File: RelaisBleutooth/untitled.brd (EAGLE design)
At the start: 160 x 100 mm, 3 parts

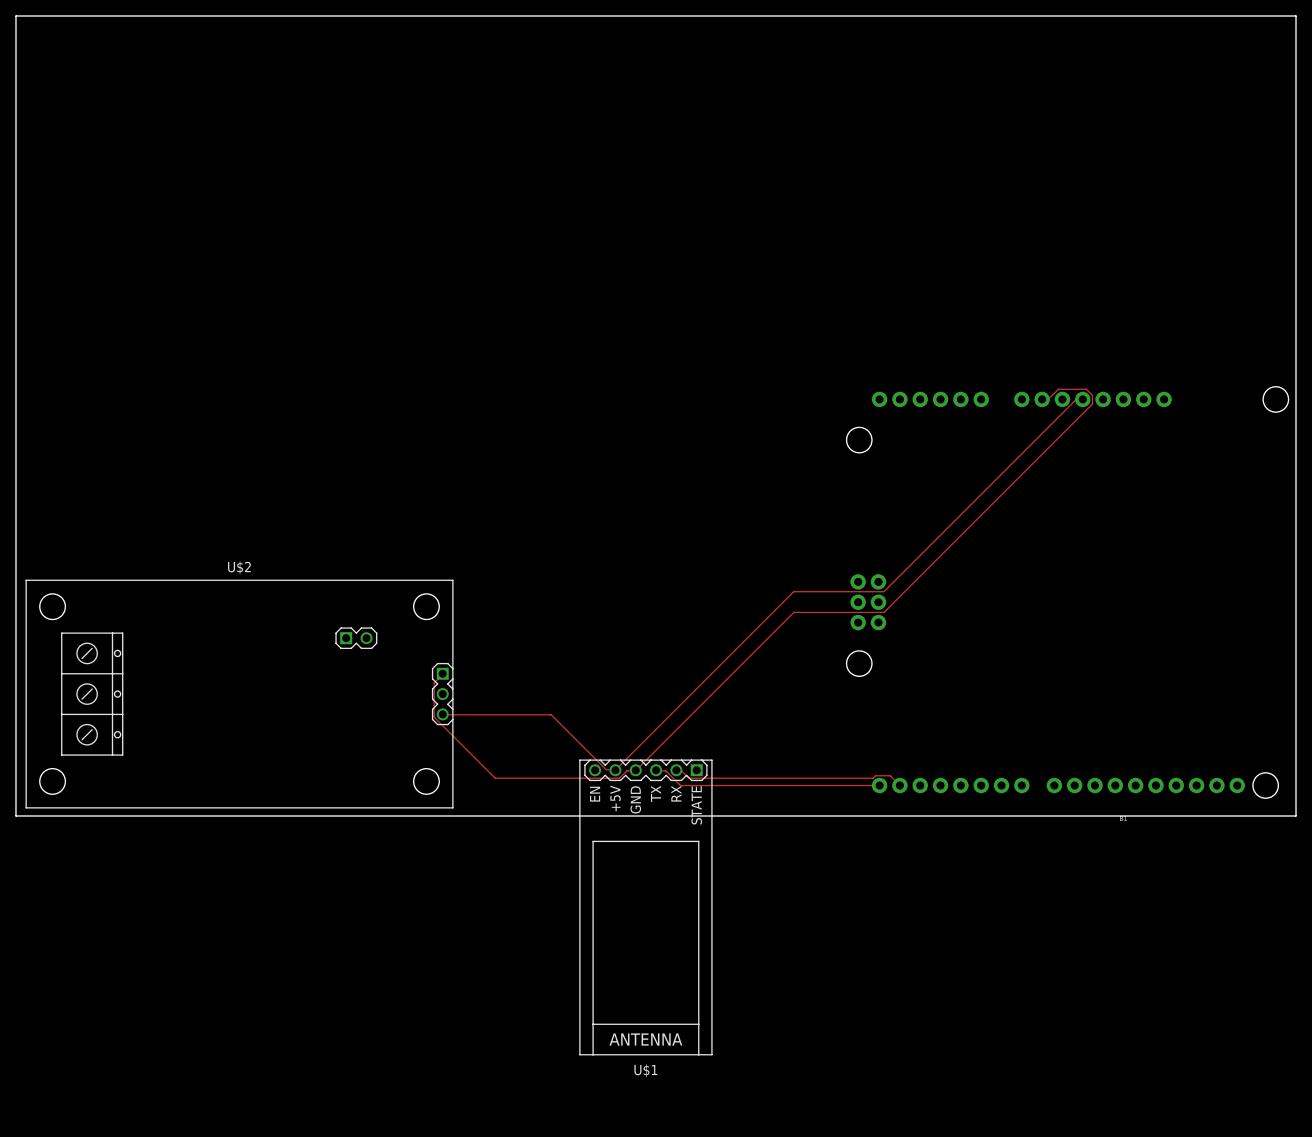
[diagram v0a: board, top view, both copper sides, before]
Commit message: Mise a jour des schema
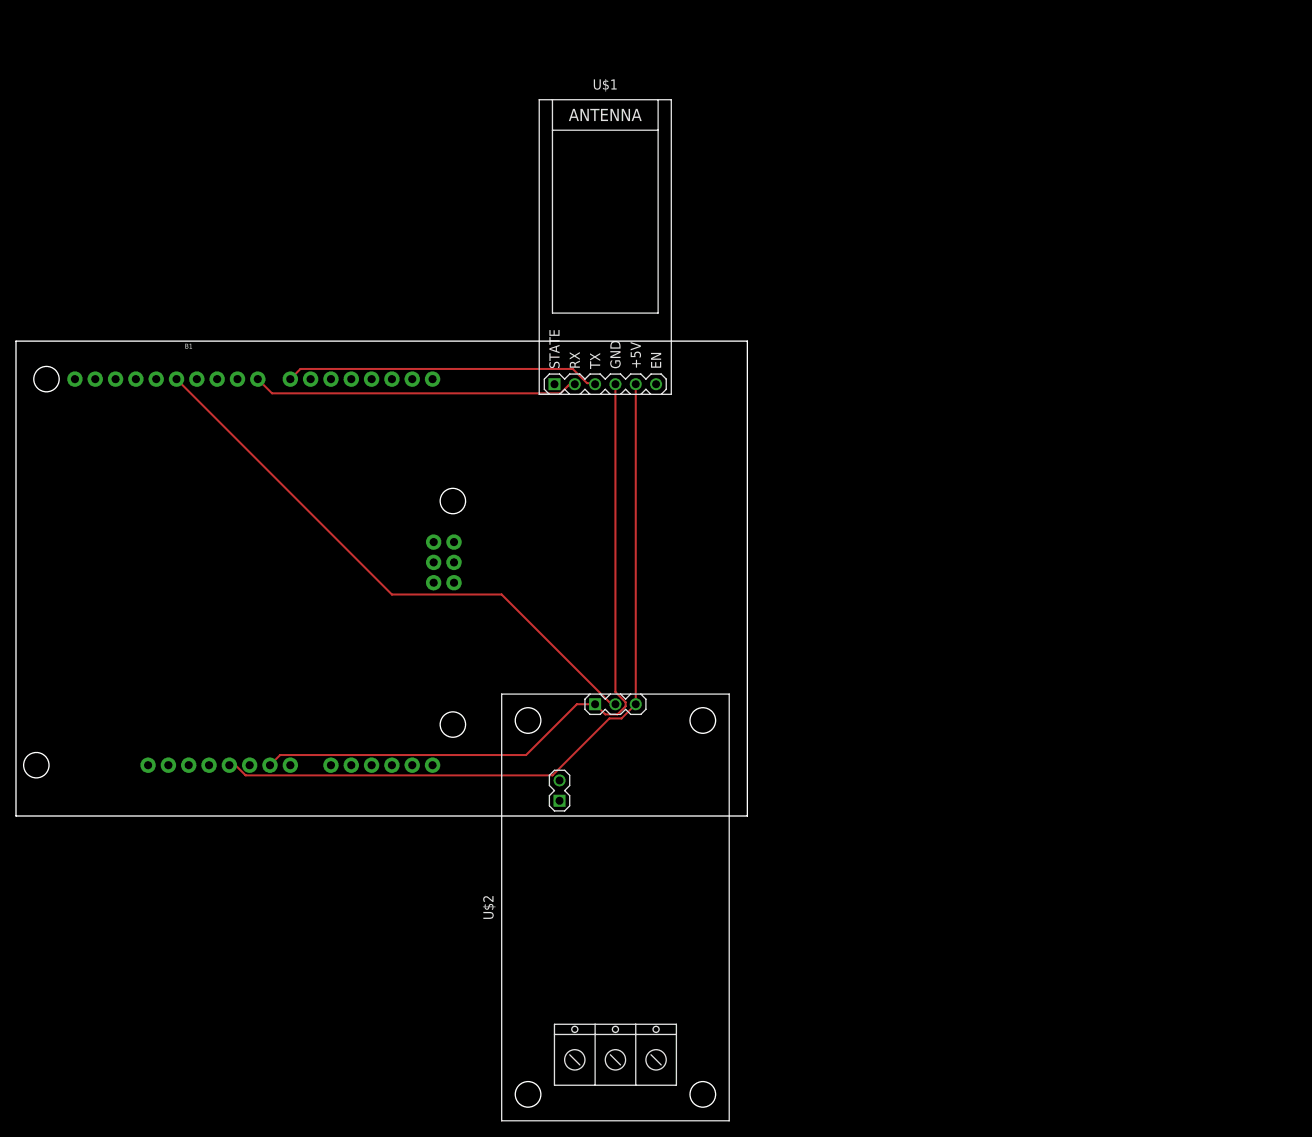
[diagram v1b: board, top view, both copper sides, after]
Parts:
- moved B1 116.9 mm to (21.6, 30.5), turned to 0 degrees
- moved U$1 82.7 mm to (73.7, 71.1), turned to 0 degrees
- moved U$2 54.0 mm to (74.9, -11.4), turned to 90 degrees
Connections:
- new net N$2: B1.D12, U$2.J1.2
- net N$4: now also B1.D7; no longer B1.D0
- net N$5: now also B1.D8; no longer B1.D1
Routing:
- net N$2: track 0.00 -> 71.7 mm
- net N$3: track 118.9 -> 89.3 mm
- net N$5: track 29.0 -> 40.9 mm
- net N$4: track 28.8 -> 39.5 mm
- net N$1: track 102.2 -> 95.0 mm
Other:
- board size 160 x 100 mm -> 91.4 x 59.4 mm
